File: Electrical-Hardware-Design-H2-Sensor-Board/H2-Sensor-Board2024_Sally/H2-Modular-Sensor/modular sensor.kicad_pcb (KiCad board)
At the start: 2 copper layers, 60 x 30 mm, 15 parts, among them J1 Conn_01x03, U1 AZ1117IH-5.0, U2 MCP6007

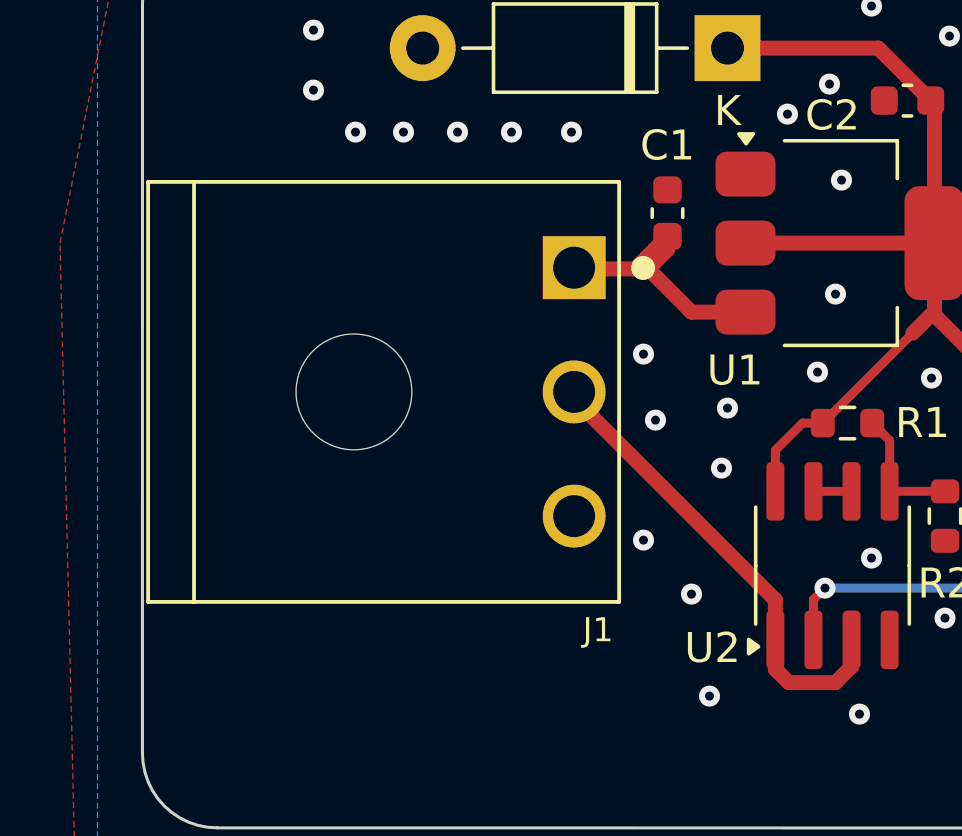
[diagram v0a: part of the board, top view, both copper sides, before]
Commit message: end-of-day update
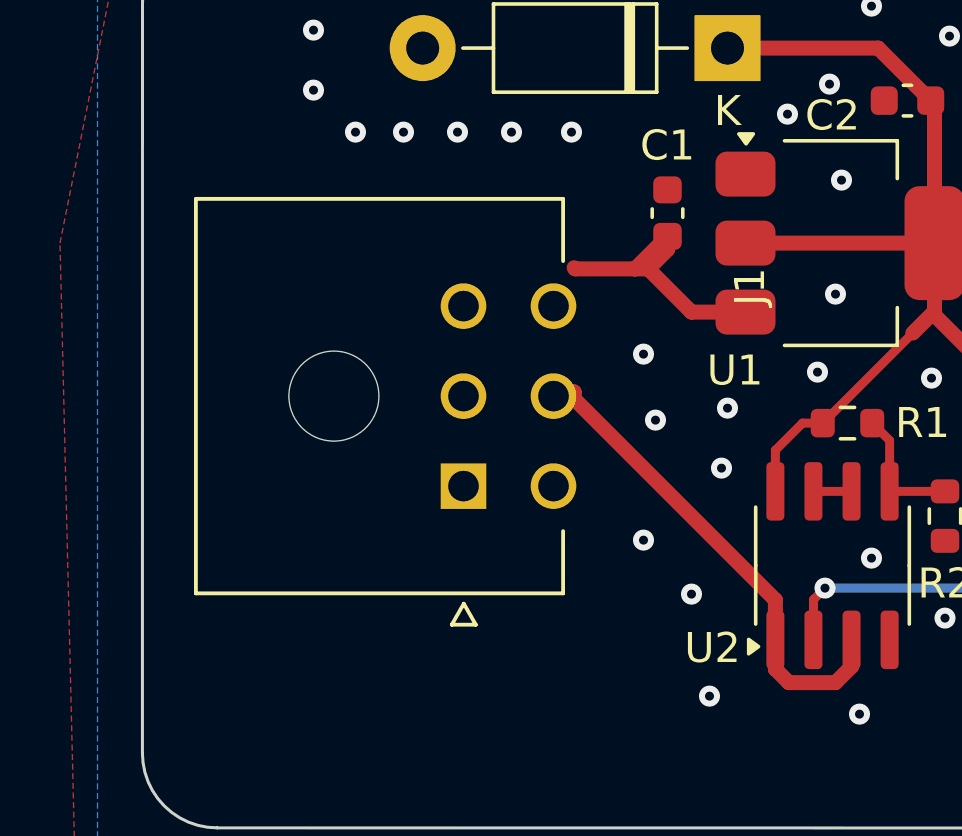
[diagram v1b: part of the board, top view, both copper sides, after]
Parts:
- J1: value Conn_01x03 -> Molex_6_Pin; footprint ecocad_lib_footprints:TE_1-770967-0 -> ecocad_lib_footprints:Molex_6_pin_RightAngle
- moved J1 4.84 mm to (119.2, 75.1)
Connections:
- J1 pad 1: /H2_PWR_unfilter -> GND
- J1 pad 2: /V_Sensed -> /H2_PWR_unfilter
- J1 pad 3: GND -> /V_Sensed
